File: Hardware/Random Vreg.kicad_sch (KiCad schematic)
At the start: 20 parts, among them J1 Conn_01x07_Male, J10 Conn_01x02_Male, J11 Conn_01x02_Male, J12 Conn_01x02_Male, J2 Conn_01x04_Male, J3 Conn_01x02_Male, J4 Conn_01x02_Male, J5 Conn_01x02_Male, J6 Conn_01x02_Male, J7 Conn_01x08_Male, J9 QWIIC_Stackable, U1 R1501J033B-T1-JE, U2 R1501J033B-T1-JE, U3 R1501J033B-T1-JE

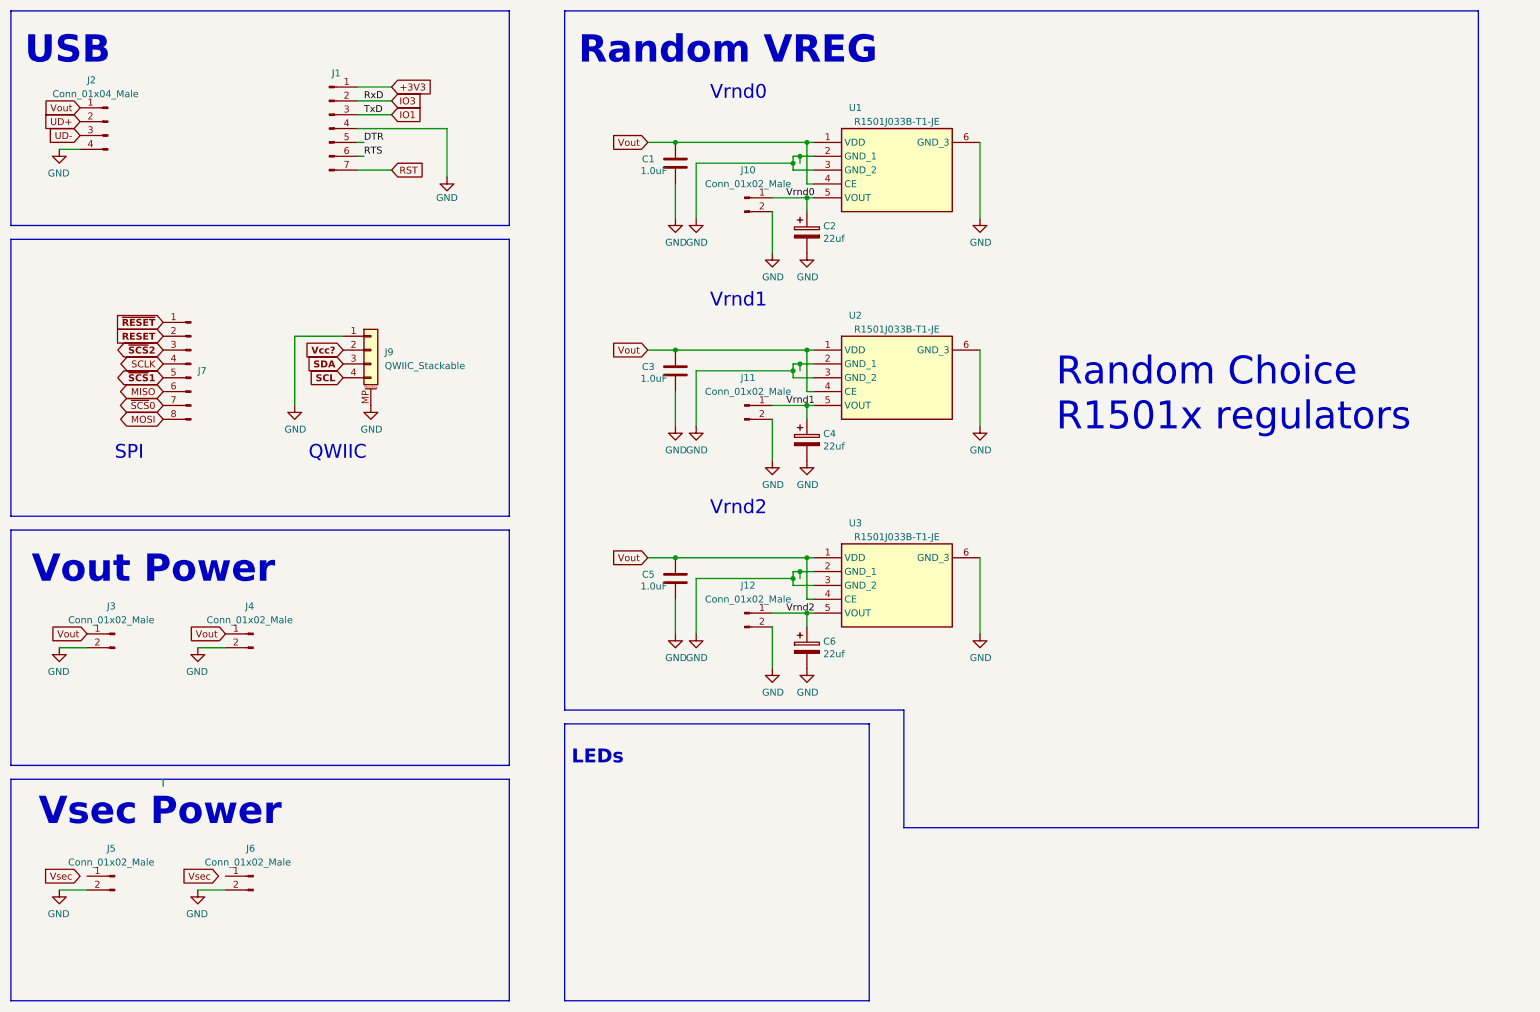
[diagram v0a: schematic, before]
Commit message: Random VREG!
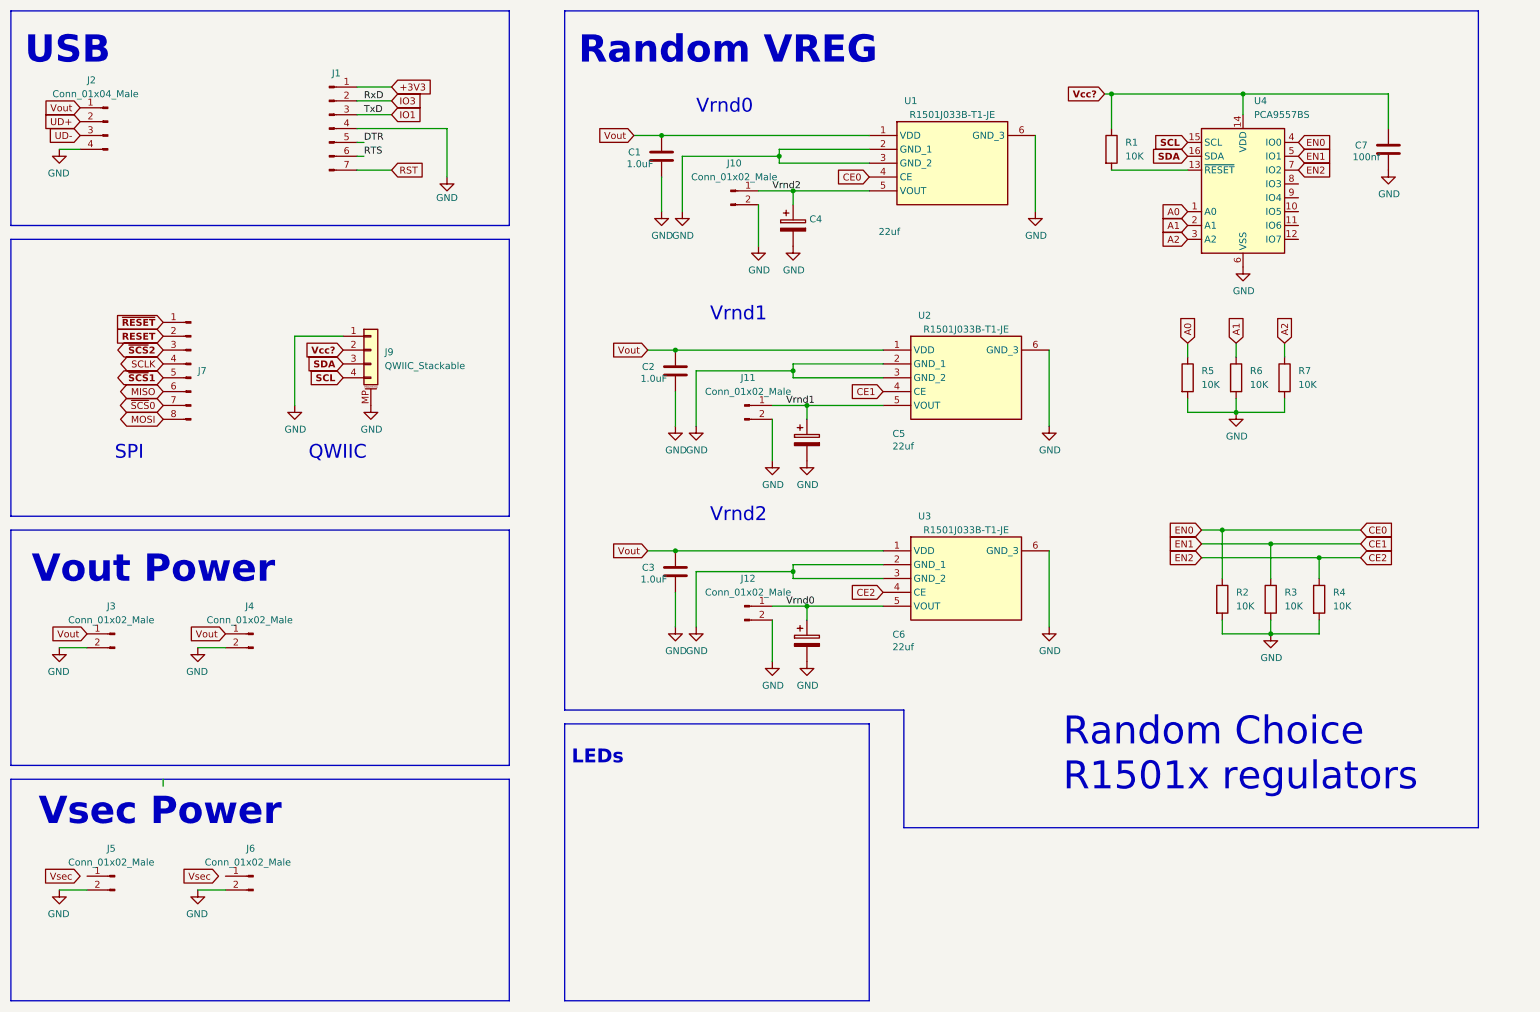
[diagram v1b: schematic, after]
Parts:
- added C7: 100nf, Capacitor_SMD:C_0603_1608Metric, symbol Device:C
- added R1, R2, R3, R4, R5, R6, R7: 10K, Resistor_SMD:R_0603_1608Metric, symbol Device:R
- added U4: PCA9557BS, Package_DFN_QFN:HVQFN-16-1EP_3x3mm_P0.5mm_EP1.5x1.5mm, symbol Interface_Expansion:PCA9557BS
- renumbered C5 to C1, C3 to C2, C1 to C3, C6 to C4, C4 to C5, C2 to C6, J12 to J10, J10 to J12, U3 to U1, U1 to U3
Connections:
- net GND: now also C7.2, R2.2, R3.2, R4.2, R5.2, R6.2, R7.2, U4.6 (VSS)
- net SCL: now also U4.15 (SCL)
- net SDA: now also U4.16 (SDA)
- net Vcc?: now also C7.1, R1.1, U4.14 (VDD)
- net Vout: no longer U1.4 (CE), U2.4 (CE), U3.4 (CE)
- new net: R1.2, U4.13 (~{RESET})
- new net A0: R5.1, U4.1 (A0)
- new net A1: R6.1, U4.2 (A1)
- new net A2: R7.1, U4.3 (A2)
- new net CE0: R2.1, U1.4 (CE), U4.4 (IO0)
- new net CE1: R3.1, U2.4 (CE), U4.5 (IO1)
- new net CE2: R4.1, U3.4 (CE), U4.7 (IO2)
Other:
- moved on the sheet: C1, C3, C4, C6, J10, J12, U1, U2, U3
